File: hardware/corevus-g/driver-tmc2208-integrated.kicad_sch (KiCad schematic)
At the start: 12 parts, among them M1 JST XH, U7 TMC2208-LA

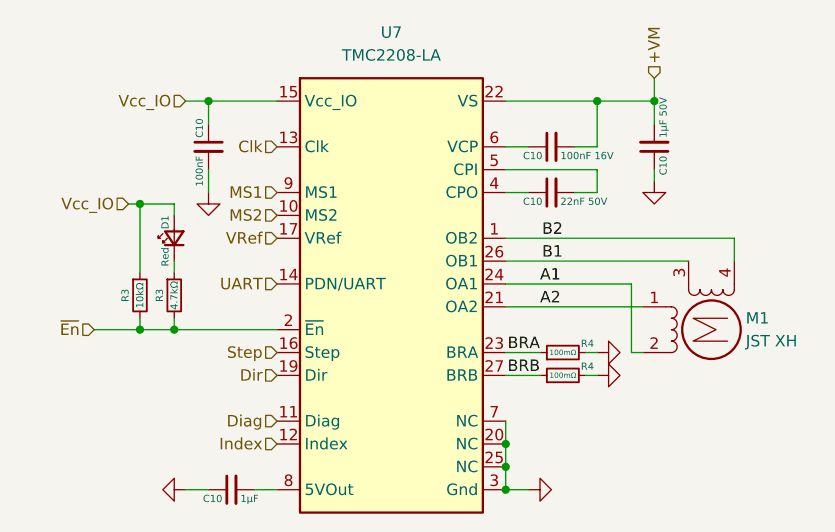
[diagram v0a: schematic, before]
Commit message: aonteuhasntoidanouidoenuthidntoehuid
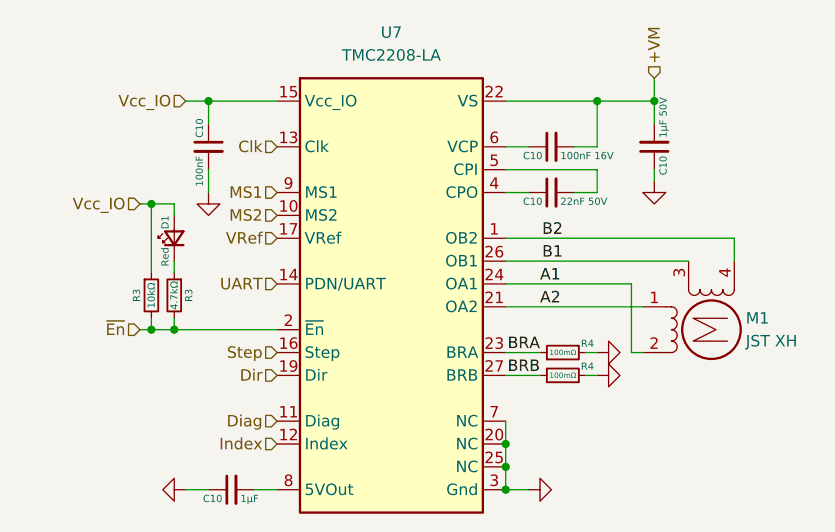
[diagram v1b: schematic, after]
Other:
- moved on the sheet: R3
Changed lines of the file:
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@@
   (junction (at 35.56 64.77) (diameter 0) (color 0 0 0 0)
   )
+  (junction (at 33.02 64.77) (diameter 0) (color 0 0 0 0)
+  )
   (junction (at 72.39 80.01) (diameter 0) (color 0 0 0 0)
   )
   (junction (at 88.9 39.37) (diameter 0) (color 0 0 0 0)
   )
-  (junction (at 31.75 64.77) (diameter 0) (color 0 0 0 0)
-  )
   (junction (at 82.55 39.37) (diameter 0) (color 0 0 0 0)
   )
@@
   (junction (at 72.39 82.55) (diameter 0) (color 0 0 0 0)
   )
-  (junction (at 31.75 50.8) (diameter 0) (color 0 0 0 0)
+  (junction (at 33.02 50.8) (diameter 0) (color 0 0 0 0)
   )
   (wire (pts (xy 72.39 49.53) (xy 74.93 49.53))
@@
     (stroke (width 0) (type default))
   )
-  (wire (pts (xy 31.75 50.8) (xy 31.75 58.42))
+  (wire (pts (xy 33.02 50.8) (xy 33.02 58.42))
     (stroke (width 0) (type default))
   )
@@
     (stroke (width 0) (type default))
   )
-  (wire (pts (xy 31.75 64.77) (xy 35.56 64.77))
+  (wire (pts (xy 31.75 64.77) (xy 33.02 64.77))
     (stroke (width 0) (type default))
   )
@@
     (stroke (width 0) (type default))
   )
-  (wire (pts (xy 31.75 50.8) (xy 35.56 50.8))
+  (wire (pts (xy 33.02 50.8) (xy 35.56 50.8))
     (stroke (width 0) (type default))
   )
@@
     (stroke (width 0) (type default))
   )
-  (wire (pts (xy 31.75 63.5) (xy 31.75 64.77))
+  (wire (pts (xy 33.02 63.5) (xy 33.02 64.77))
     (stroke (width 0) (type default))
   )
@@
     (stroke (width 0) (type default))
   )
-  (wire (pts (xy 26.67 64.77) (xy 31.75 64.77))
-    (stroke (width 0) (type default))
-  )
   (wire (pts (xy 82.55 46.99) (xy 82.55 49.53))
     (stroke (width 0) (type default))
@@
     (stroke (width 0) (type default))
   )
-  (wire (pts (xy 30.48 50.8) (xy 31.75 50.8))
+  (wire (pts (xy 31.75 50.8) (xy 33.02 50.8))
     (stroke (width 0) (type default))
   )
@@
   )
   (wire (pts (xy 72.39 67.31) (xy 76.2 67.31))
+    (stroke (width 0) (type default))
+  )
+  (wire (pts (xy 33.02 64.77) (xy 35.56 64.77))
     (stroke (width 0) (type default))
   )
@@
     (effects (font (size 1.27 1.27)) (justify left bottom))
   )
-  (hierarchical_label "Vcc_IO" (shape input) (at 30.48 50.8 180) (fields_autoplaced)
+  (hierarchical_label "Vcc_IO" (shape input) (at 31.75 50.8 180) (fields_autoplaced)
     (effects (font (size 1.27 1.27)) (justify right))
   )
@@
     (effects (font (size 1.27 1.27)) (justify right))
   )
-  (hierarchical_label "~{En}" (shape input) (at 26.67 64.77 180) (fields_autoplaced)
+  (hierarchical_label "~{En}" (shape input) (at 31.75 64.77 180) (fields_autoplaced)
     (effects (font (size 1.27 1.27)) (justify right))
   )
@@
     )
   )
-  (symbol (lib_id "Device:R_Small") (at 35.56 60.96 0) (unit 1)
+  (symbol (lib_id "Device:R_Small") (at 35.56 60.96 0) (mirror y) (unit 1)
     (in_bom yes) (on_board yes) (dnp no)
-    (property "Reference" "R3" (at 33.93 60.96 90)
+    (property "Reference" "R3" (at 37.19 60.96 90)
       (effects (font (size 0.8 0.8)))
     )
@@
     )
   )
-  (symbol (lib_id "Device:R_Small") (at 31.75 60.96 0) (unit 1)
+  (symbol (lib_id "Device:R_Small") (at 33.02 60.96 0) (unit 1)
     (in_bom yes) (on_board yes) (dnp no)
-    (property "Reference" "R3" (at 30.12 60.96 90)
+    (property "Reference" "R3" (at 31.39 60.96 90)
       (effects (font (size 0.8 0.8)))
     )
-    (property "Value" "10kΩ" (at 31.75 60.96 90)
+    (property "Value" "10kΩ" (at 33.02 60.96 90)
       (effects (font (size 0.8 0.8)))
     )
-    (property "Footprint" "AlphaLib:0402R" (at 31.75 60.96 0)
-      (effects (font (size 1.27 1.27)) hide)
-    )
-    (property "Datasheet" "~" (at 31.75 60.96 0)
-      (effects (font (size 1.27 1.27)) hide)
-    )
+    (property "Footprint" "AlphaLib:0402R" (at 33.02 60.96 0)
+      (effects (font (size 1.27 1.27)) hide)
+    )
+    (property "Datasheet" "~" (at 33.02 60.96 0)
+      (effects (font (size 1.27 1.27)) hide)
+    )

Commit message: v0.4 mostly complete, board needs minor revisions (e.g. pin swap)
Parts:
- M1: footprint corevus:JST_XH_1x04-Side -> corevus:JST_XH_1x04
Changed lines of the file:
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@@
       )
       (project "corevus-g"
-        (path "/1a565782-f217-442e-b118-196625f31c53"
-          (reference "R96") (unit 1)
-        )
-        (path "/1a565782-f217-442e-b118-196625f31c53/09bb4a8f-8694-4b82-8e1f-fabe3bd11ec7"
-          (reference "R98") (unit 1)
-        )
-        (path "/1a565782-f217-442e-b118-196625f31c53/d34aeff3-da22-4edc-92e0-1591d6117dbc"
-          (reference "R99") (unit 1)
-        )
         (path "/1a565782-f217-442e-b118-196625f31c53/972ca71f-1c40-4278-8cb4-2b520c3e8975"
           (reference "R22") (unit 1)
@@
       (effects (font (size 1.27 1.27)) (justify right))
     )
-    (property "Footprint" "corevus:JST_XH_1x04-Side" (at 95.504 65.024 0)
+    (property "Footprint" "corevus:JST_XH_1x04" (at 95.504 65.024 0)
       (effects (font (size 1.27 1.27)) hide)
     )
@@
       )
       (project "corevus-g"
-        (path "/1a565782-f217-442e-b118-196625f31c53"
-          (reference "R96") (unit 1)
-        )
-        (path "/1a565782-f217-442e-b118-196625f31c53/09bb4a8f-8694-4b82-8e1f-fabe3bd11ec7"
-          (reference "R98") (unit 1)
-        )
-        (path "/1a565782-f217-442e-b118-196625f31c53/d34aeff3-da22-4edc-92e0-1591d6117dbc"
-          (reference "R99") (unit 1)
-        )
         (path "/1a565782-f217-442e-b118-196625f31c53/972ca71f-1c40-4278-8cb4-2b520c3e8975"
           (reference "R97") (unit 1)
@@
       )
       (project "corevus-g"
-        (path "/1a565782-f217-442e-b118-196625f31c53"
-          (reference "D18") (unit 1)
-        )
-        (path "/1a565782-f217-442e-b118-196625f31c53/09bb4a8f-8694-4b82-8e1f-fabe3bd11ec7"
-          (reference "D19") (unit 1)
-        )
-        (path "/1a565782-f217-442e-b118-196625f31c53/d34aeff3-da22-4edc-92e0-1591d6117dbc"
-          (reference "D20") (unit 1)
-        )
         (path "/1a565782-f217-442e-b118-196625f31c53/972ca71f-1c40-4278-8cb4-2b520c3e8975"
           (reference "D21") (unit 1)

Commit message: CvG v0.4 complete, now updating documentation
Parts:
- C10: LCSC C19666 -> (none)
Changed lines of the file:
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@@
       (effects (font (size 1.27 1.27)) hide)
     )
-    (property "LCSC" "C19666" (at 41.91 82.55 90)
+    (property "LCSC" "" (at 41.91 82.55 90)
       (effects (font (size 1.27 1.27)) hide)
     )
